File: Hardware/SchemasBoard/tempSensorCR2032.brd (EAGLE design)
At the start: 22.2 x 24.1 mm, 9 parts, among them IC1 DS1820

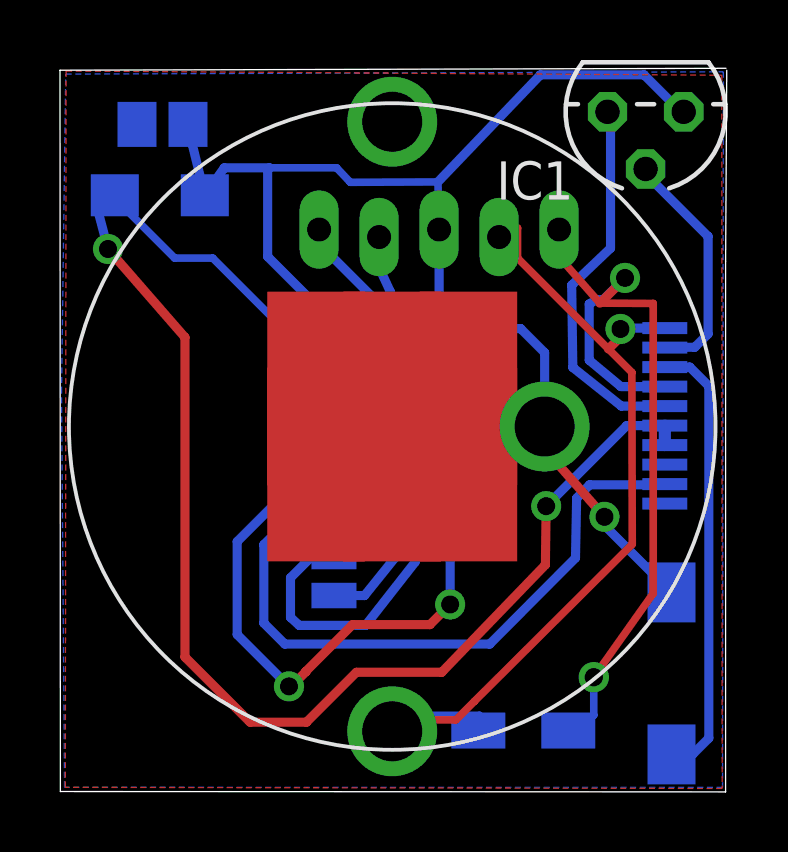
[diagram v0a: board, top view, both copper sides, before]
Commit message: aa
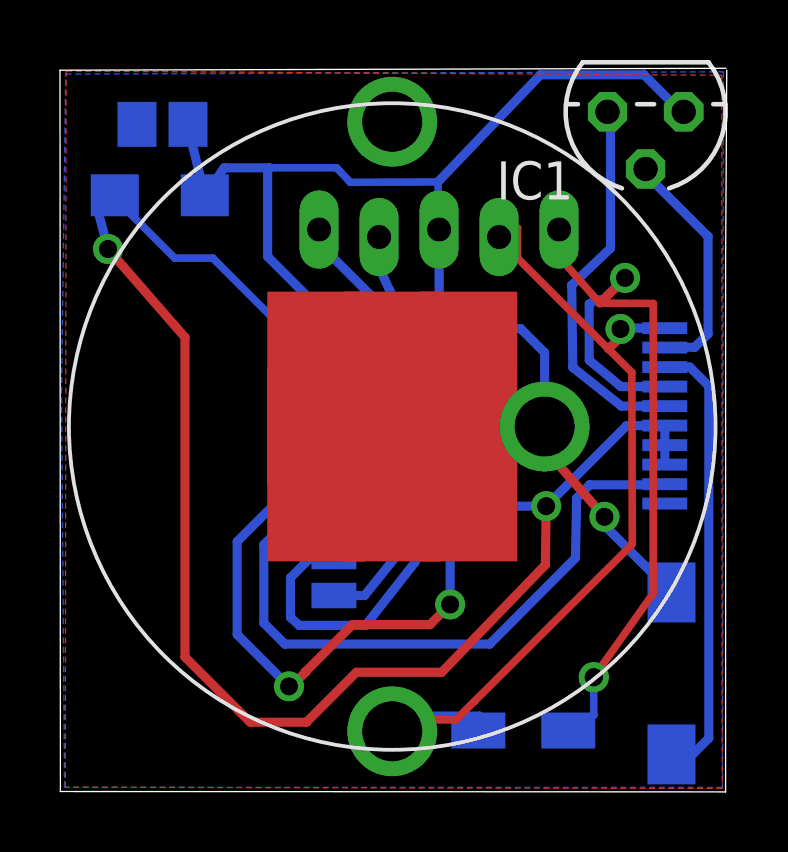
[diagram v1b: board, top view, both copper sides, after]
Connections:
- net N$4: now also U$2.15, U$2.8
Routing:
- net N$4: track 50.9 -> 57.6 mm
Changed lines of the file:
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@@
 <contactref element="U$1" pad="VDD"/>
 <contactref element="C2" pad="+"/>
-<wire x1="20.1477" y1="11.5472" x2="20.1477" y2="12.1972" width="0.4064" layer="16"/>
+<wire x1="20.1477" y1="11.5472" x2="20.1477" y2="12.1972" width="0.3048" layer="16"/>
 <wire x1="5.08" y1="17.78" x2="8.89" y2="13.97" width="0.254" layer="16"/>
 <wire x1="3.81" y1="17.78" x2="5.08" y2="17.78" width="0.254" layer="16"/>
@@
 <wire x1="1.5875" y1="18.0848" x2="1.2065" y2="19.534" width="0.3048" layer="16"/>
 <wire x1="1.2065" y1="19.534" x2="1.8147" y2="19.8755" width="0.3048" layer="16"/>
+<contactref element="U$2" pad="8"/>
+<contactref element="U$2" pad="15"/>
+<wire x1="16.1925" y1="9.5123" x2="14.1605" y2="9.5123" width="0.3048" layer="16"/>
+<wire x1="14.1605" y1="9.5123" x2="14.1605" y2="12.2047" width="0.3048" layer="16"/>
+<wire x1="14.1605" y1="12.2047" x2="12.8977" y2="12.2047" width="0.3048" layer="16"/>
+<wire x1="12.8977" y1="12.2047" x2="12.8977" y2="12.1972" width="0.3048" layer="16"/>
+<wire x1="20.1477" y1="11.5472" x2="20.1477" y2="10.8972" width="0.3048" layer="16"/>
 </signal>
 <signal name="N$5">
